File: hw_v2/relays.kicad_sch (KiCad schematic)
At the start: 26 parts, among them J10 Conn_01x01, J11 Conn_01x01, J2 Conn_01x01, J3 Conn_01x01, Q4 SS8050, Q5 SS8050, Q6 AO3400A, Q7 AO3400A, U18 VNLD5090, U5 TPL7407LAPWR

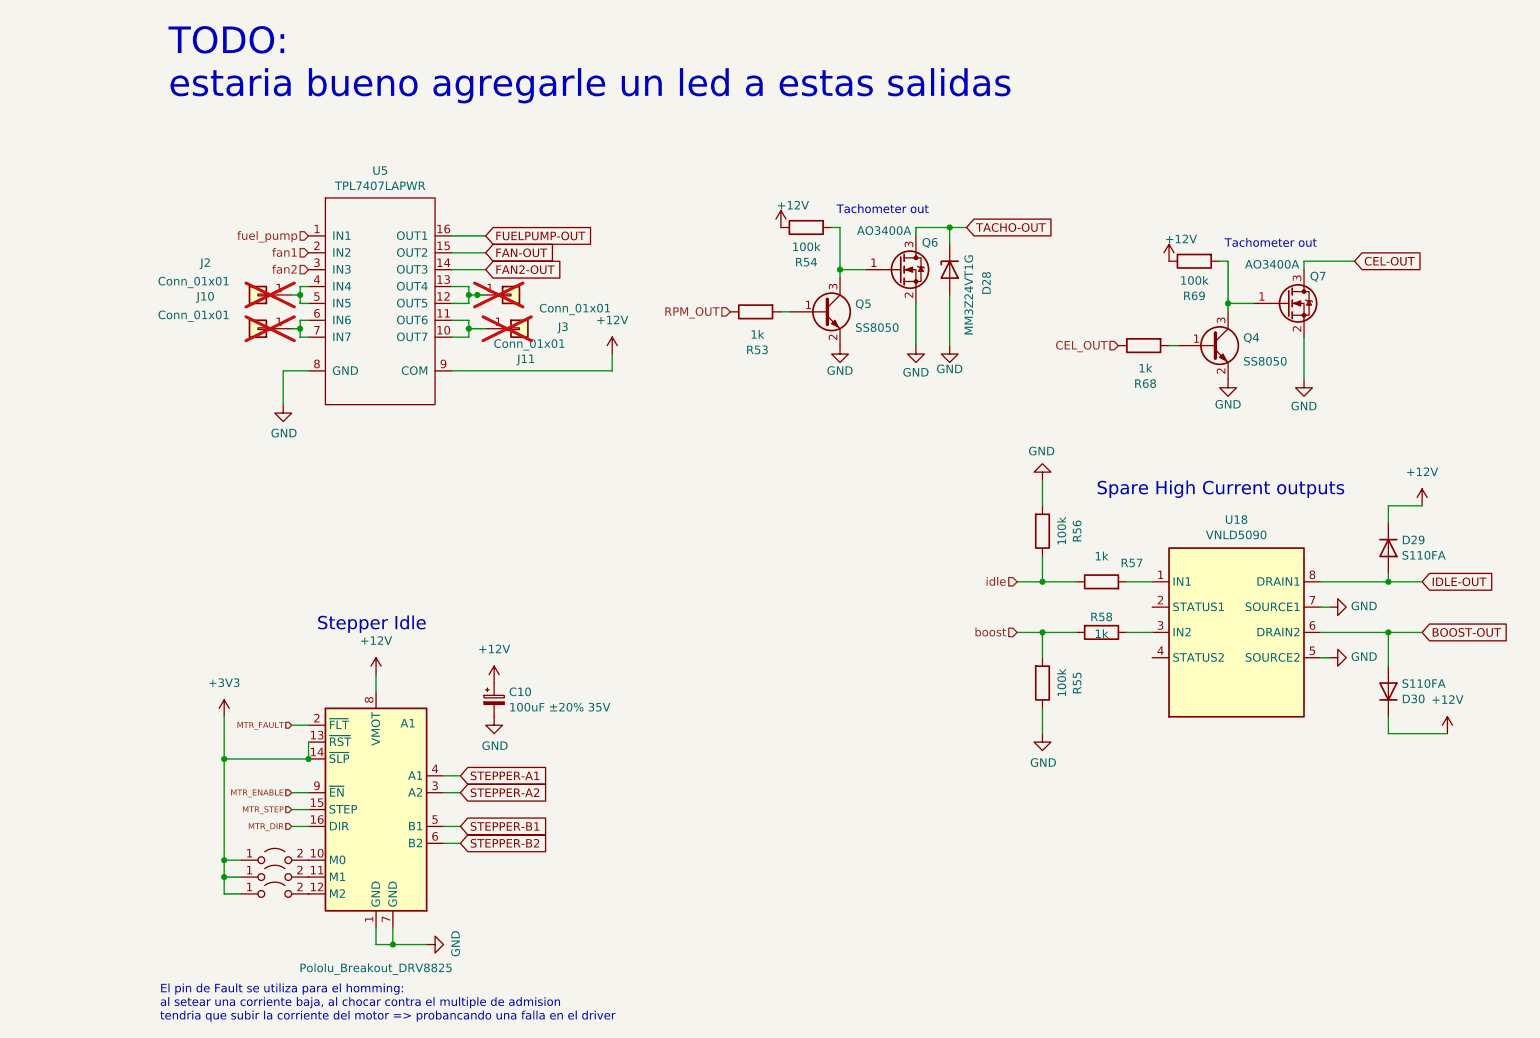
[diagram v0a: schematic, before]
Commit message: hw v2
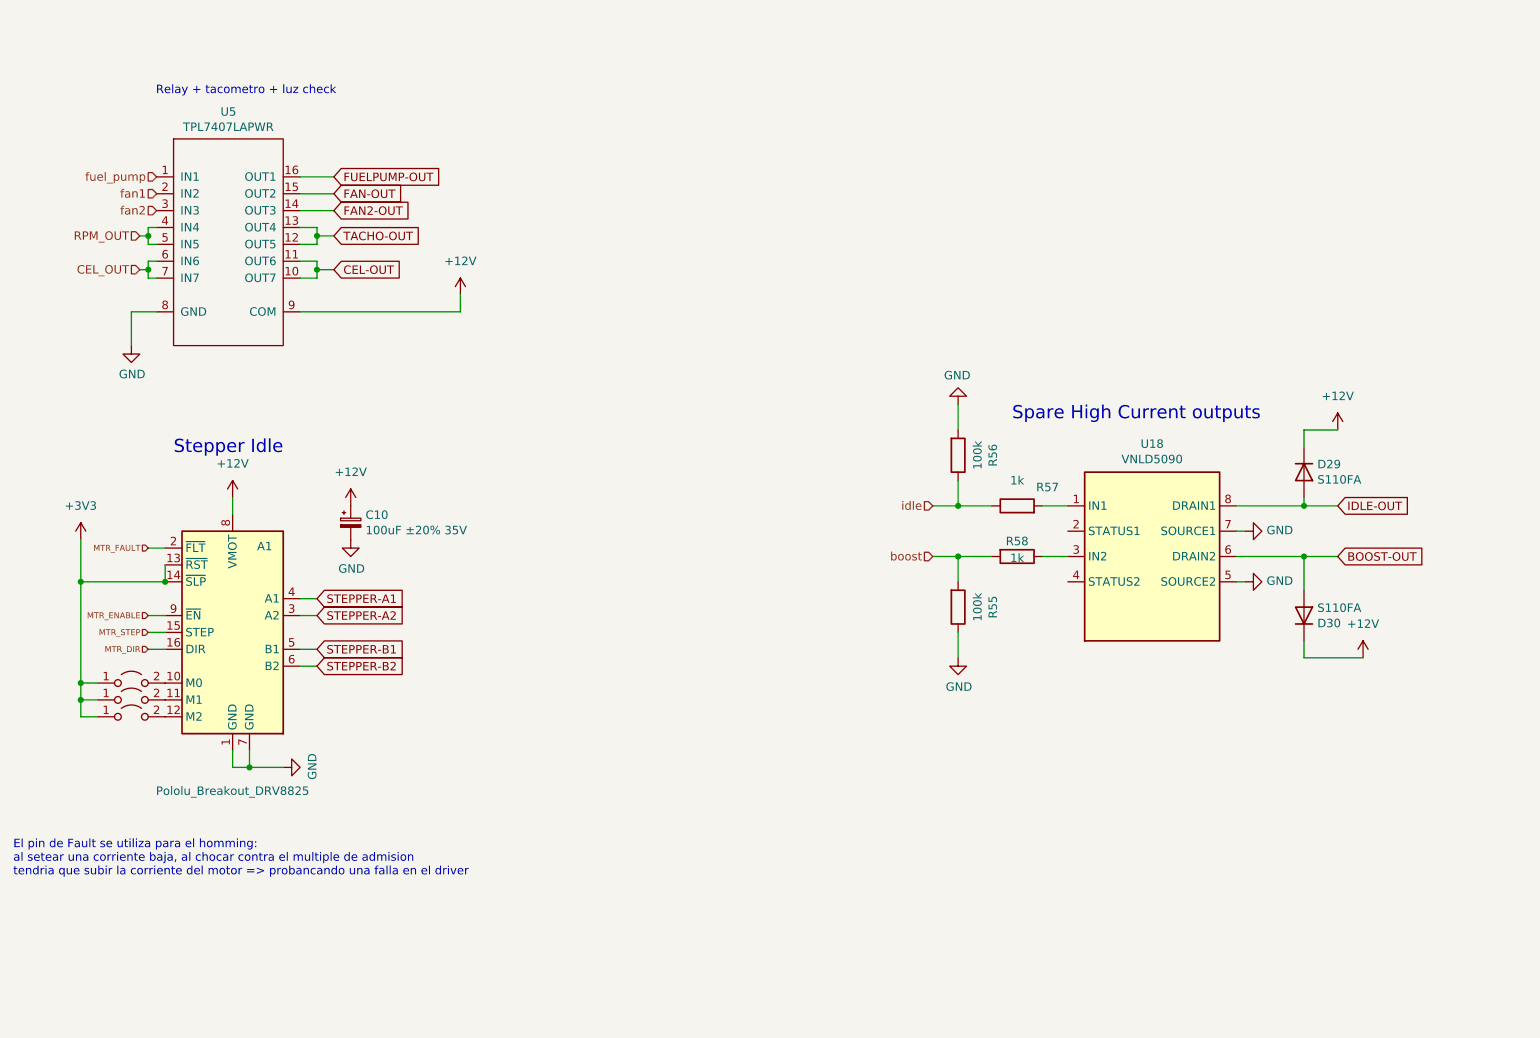
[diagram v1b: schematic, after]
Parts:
- removed D28: MM3Z24VT1G, Diode_SMD:D_SOD-323, symbol Device:D_Zener
- removed J10, J11, J2, J3: Conn_01x01, TestPoint:TestPoint_THTPad_2.0x2.0mm_Drill1.0mm, symbol Connector_Generic:Conn_01x01
- removed Q4, Q5: SS8050, Package_TO_SOT_SMD:SOT-23, symbol Transistor_BJT:2N3055
- removed Q6, Q7: AO3400A, Package_TO_SOT_SMD:SOT-23, symbol Transistor_FET:AO3400A
- removed R53, R68: 1k, Resistor_SMD:R_0603_1608Metric, symbol Device:R
- removed R54, R69: 100k, Resistor_SMD:R_0603_1608Metric, symbol Device:R
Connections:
- net CEL-OUT: now also U5.10 (OUT7), U5.11 (OUT6)
- net CEL_OUT: now also U5.6 (IN6), U5.7 (IN7)
- net RPM_OUT: now also U5.4 (IN4), U5.5 (IN5)
- net TACHO-OUT: now also U5.12 (OUT5), U5.13 (OUT4)
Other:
- note added: "Relay + tacometro + luz check"
- note removed: "TODO: estaria bueno agregarle un led a estas salidas"
- note removed: "Tachometer out"
- moved on the sheet: A1, C10, D29, D30, R55, R56, R57, R58, U18, U5
